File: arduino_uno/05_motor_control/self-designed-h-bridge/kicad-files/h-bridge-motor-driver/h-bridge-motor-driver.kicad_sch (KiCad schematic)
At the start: 18 parts, among them J1 Conn_01x05_Pin, J2 Conn_01x02_Pin, J3 2601-3102, J4 2601-3102, Q1 IRF9540N, Q2 IRLIZ44N, Q3 IRF9540N, Q4 IRLIZ44N, Q5 BC547, Q6 BC547

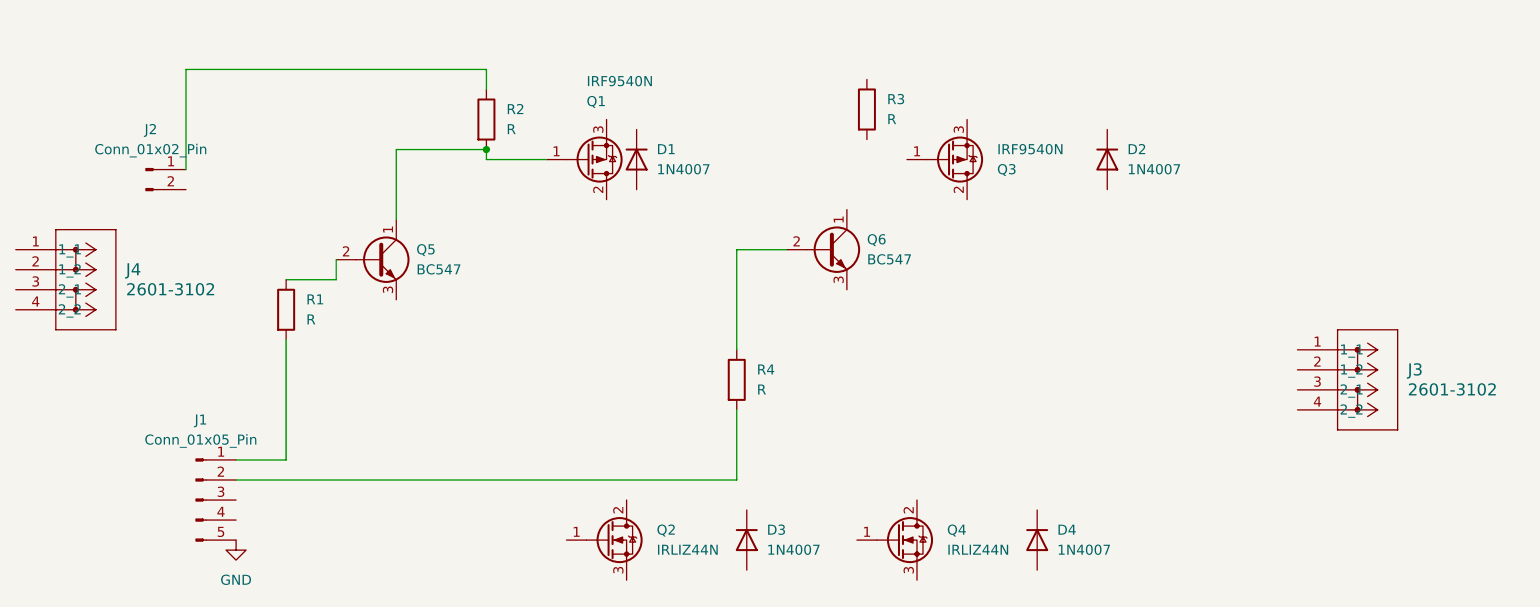
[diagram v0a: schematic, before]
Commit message: rework schematic
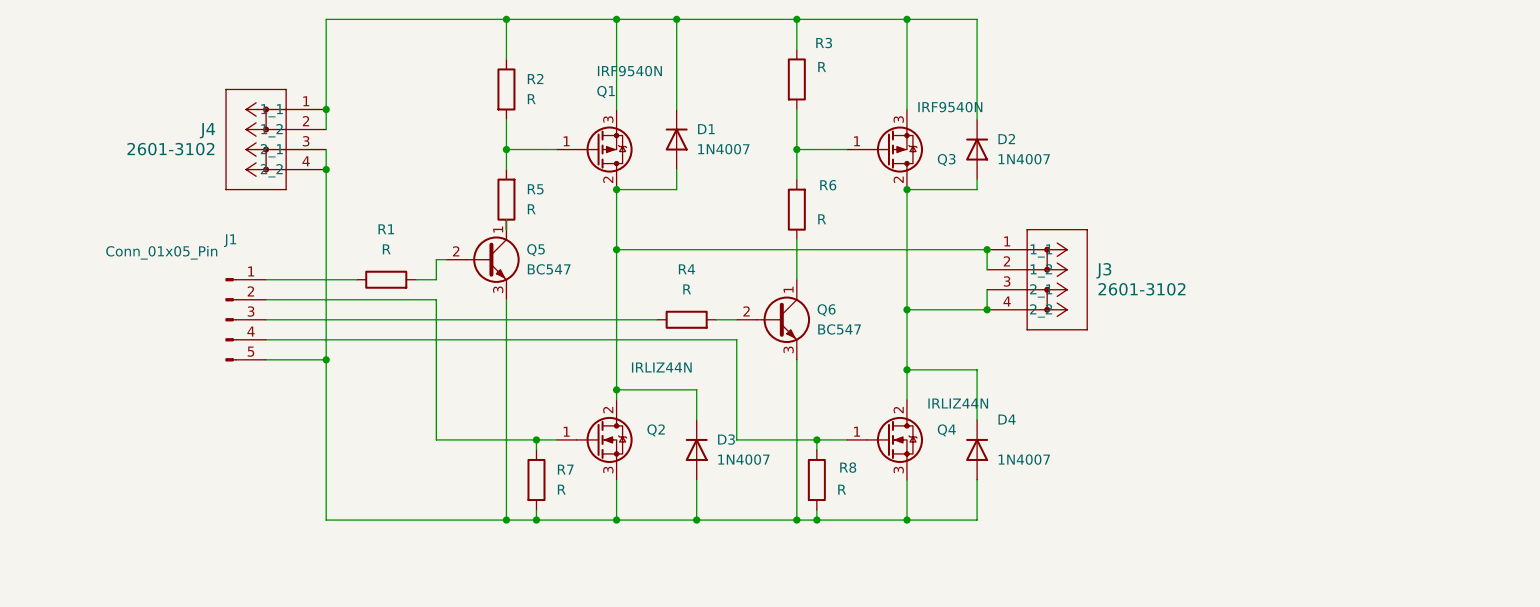
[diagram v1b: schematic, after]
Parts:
- removed J2: Conn_01x02_Pin, symbol Connector:Conn_01x02_Pin
- added R5, R6, R7, R8: R, symbol Device:R
- J3, J4: footprint CONN2_2601-3102_WAG -> WAGO 2601-3102:CONN2_2601-3102_WAG
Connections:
- net GND is gone; now on an unnamed net: J1.5 (Pin_5)
- net at D2.1 (K): now also D1.1 (K), J4.1 (1_1), J4.2 (1_2), Q1.3 (S), Q3.3 (S), R2.1, R3.1
- net at D2.2 (A): now also D4.1 (K), J3.3 (2_1), J3.4 (2_2), Q3.2 (D), Q4.2 (D)
- net at Q3.1 (G): now also R3.2, R6.2
- net at Q4.1 (G): now also J1.4 (Pin_4), R8.1
- net at Q4.3 (S): now also D3.2 (A), D4.2 (A), J4.3 (2_1), J4.4 (2_2), Q2.3 (S), Q5.3 (E), Q6.3 (E), R7.2, R8.2
- net at Q1.1 (G), R2.2: now also R5.2; no longer Q5.1 (C)
- net at Q5.2 (B): now also R1.2; no longer R1.1
- net at J1.1 (Pin_1): now also R1.1; no longer R1.2
- net at J1.2 (Pin_2): now also Q2.1 (G), R7.1; no longer R4.2
- net at J1.3 (Pin_3): now also R4.1
- net at Q6.1 (C): now also R6.1
- net at Q6.2 (B): now also R4.2; no longer R4.1
- net at Q2.2 (D): now also D1.2 (A), D3.1 (K), J3.1 (1_1), J3.2 (1_2), Q1.2 (D)
- new net: Q5.1 (C), R5.1
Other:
- moved on the sheet: D1, D2, D3, D4, J1, J3, J4, Q1, Q2, Q3, Q4, Q5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
